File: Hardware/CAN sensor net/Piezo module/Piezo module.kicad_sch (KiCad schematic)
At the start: 40 parts, among them SW1 SW_Push, SW2 SW_SPDT, U1 SN65HVD230, U2 STM32F103C8Tx, U3 W25Q32FVSSIG, Y1 16MHz

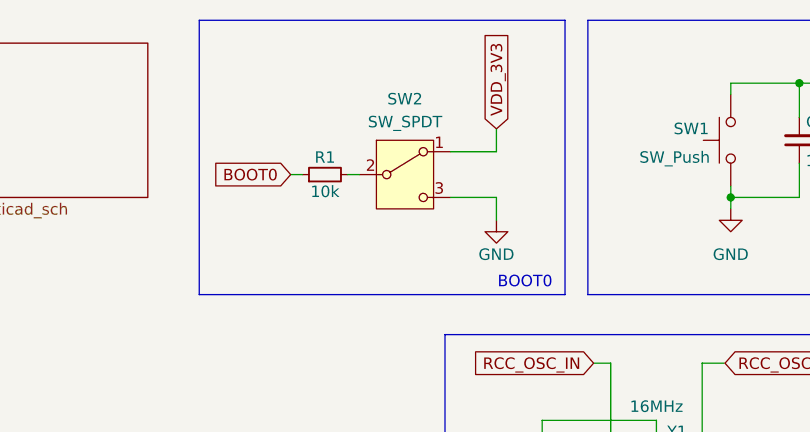
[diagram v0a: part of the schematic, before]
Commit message: Bugfix
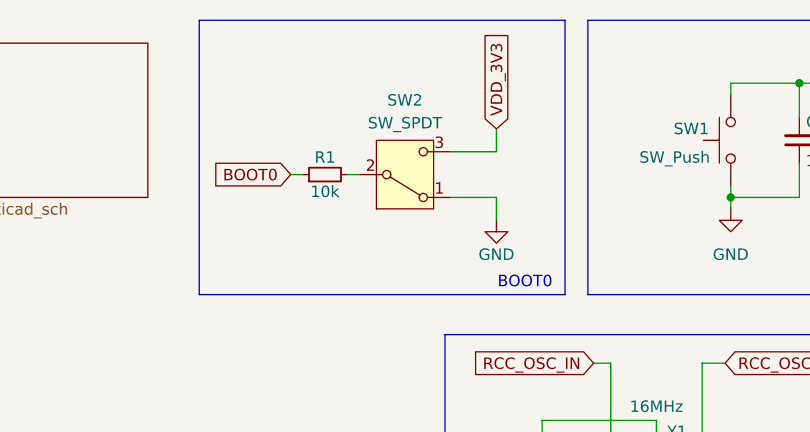
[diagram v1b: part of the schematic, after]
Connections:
- net GND: now also SW2.1 (A); no longer SW2.3 (C)
- net VDD_3V3: now also SW2.3 (C); no longer SW2.1 (A)
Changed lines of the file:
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@@
 		(lib_id "Switch:SW_SPDT")
 		(at 130.81 33.02 0)
+		(mirror x)
 		(unit 1)
 		(exclude_from_sim no)
@@
 		(dnp no)
 		(property "Reference" "SW2"
-			(at 130.81 24.638 0)
+			(at 130.81 24.765 0)
 			(effects
 				(font
@@
 		)
 		(property "Value" "SW_SPDT"
-			(at 130.81 27.178 0)
+			(at 130.81 27.305 0)
 			(effects
 				(font
@@
 		)
 		(property "Datasheet" "~"
-			(at 130.81 40.64 0)
+			(at 130.81 25.4 0)
 			(effects
 				(font
